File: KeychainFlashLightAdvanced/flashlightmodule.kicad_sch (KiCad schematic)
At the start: 4 parts, among them SW1 SW_DPST_x2

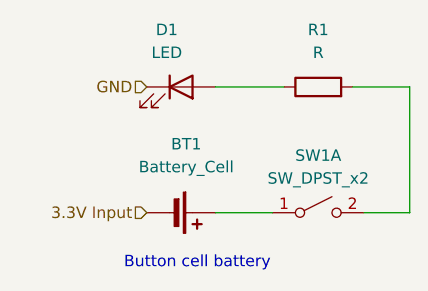
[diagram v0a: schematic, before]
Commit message: cleanup
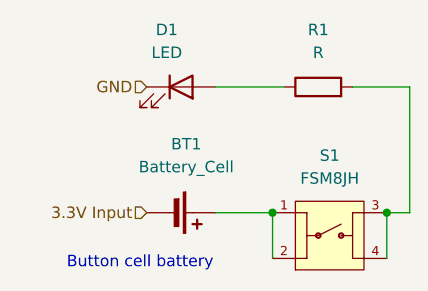
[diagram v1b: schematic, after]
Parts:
- removed SW1: SW_DPST_x2, Button_Switch_THT:SW_Tactile_Straight_KSA0Axx1LFTR, symbol Switch:SW_DPST_x2
- added S1: FSM8JH, FSM8JH:SW_FSM8JH, symbol FSM8JH:FSM8JH
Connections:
- net at BT1.1 (+): now also S1.1, S1.2
- net at R1.2: now also S1.3, S1.4
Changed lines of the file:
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@@
     (comment 1 "Made By: Casper Tak")
   )
+  (junction (at 156.21 106.68) (diameter 0) (color 0 0 0 0)
+  )
+  (junction (at 168.91 106.68) (diameter 0) (color 0 0 0 0)
+  )
   (wire (pts (xy 149.86 106.68) (xy 156.21 106.68))
+    (stroke (width 0) (type default))
+  )
+  (wire (pts (xy 168.91 106.68) (xy 168.91 111.76))
     (stroke (width 0) (type default))
   )
@@
     (stroke (width 0) (type default))
   )
+  (wire (pts (xy 156.21 106.68) (xy 156.21 111.76))
+    (stroke (width 0) (type default))
+  )
   (wire (pts (xy 171.45 92.71) (xy 171.45 106.68))
     (stroke (width 0) (type default))
   )
-  (wire (pts (xy 171.45 106.68) (xy 166.37 106.68))
+  (wire (pts (xy 171.45 106.68) (xy 168.91 106.68))
     (stroke (width 0) (type default))
   )
@@
     (stroke (width 0) (type default))
   )
-  (text "Button cell battery" (at 139.7 113.03 0)
+  (text "Button cell battery" (at 133.35 113.03 0)
     (effects (font (size 1.27 1.27)) (justify left bottom))
   )
@@
   (hierarchical_label "GND" (shape input) (at 142.24 92.71 180) (fields_autoplaced)
     (effects (font (size 1.27 1.27)) (justify right))
+  )
+  (symbol (lib_id "FSM8JH:FSM8JH") (at 162.56 109.22 0) (unit 1)
+    (in_bom yes) (on_board yes) (dnp no) (fields_autoplaced)
+    (property "Reference" "S1" (at 162.56 100.33 0)
+      (effects (font (size 1.27 1.27)))
+    )
+    (property "Value" "FSM8JH" (at 162.56 102.87 0)
+      (effects (font (size 1.27 1.27)))
+    )
+    (property "Footprint" "FSM8JH:SW_FSM8JH" (at 162.56 109.22 0)
+      (effects (font (size 1.27 1.27)) (justify bottom) hide)
+    )
+    (property "Datasheet" "" (at 162.56 109.22 0)
+      (effects (font (size 1.27 1.27)) hide)
+    )
+    (property "MF" "TE Connectivity" (at 162.56 109.22 0)
+      (effects (font (size 1.27 1.27)) (justify bottom) hide)
+    )
+    (property "Description" "\nSwitch,Pushbutton,Tactile,SPST,Thru Hole,Vertical,6MM,Black | TE Connectivity FSM8JH\n" (at 162.56 109.22 0)
+      (effects (font (size 1.27 1.27)) (justify bottom) hide)
+    )
+    (property "Package" "None" (at 162.56 109.22 0)
+      (effects (font (size 1.27 1.27)) (justify bottom) hide)
+    )
+    (property "Price" "None" (at 162.56 109.22 0)
+      (effects (font (size 1.27 1.27)) (justify bottom) hide)
+    )
+    (property "Check_prices" "https://www.snapeda.com/parts/FSM8JH/TE+Connectivity+ALCOSWITCH+Switches/view-part/?ref=eda" (at 162.56 109.22 0)
+      (effects (font (size 1.27 1.27)) (justify bottom) hide)
+    )
+    (property "STANDARD" "MANUFACTURER RECOMMENDATIONS" (at 162.56 109.22 0)
+      (effects (font (size 1.27 1.27)) (justify bottom) hide)
+    )
+    (property "PARTREV" "C10" (at 162.56 109.22 0)
+      (effects (font (size 1.27 1.27)) (justify bottom) hide)
+    )
+    (property "SnapEDA_Link" "https://www.snapeda.com/parts/FSM8JH/TE+Connectivity+ALCOSWITCH+Switches/view-part/?ref=snap" (at 162.56 109.22 0)
+      (effects (font (size 1.27 1.27)) (justify bottom) hide)
+    )
+    (property "MP" "FSM8JH" (at 162.56 109.22 0)
+      (effects (font (size 1.27 1.27)) (justify bottom) hide)
+    )
+    (property "Availability" "In Stock" (at 162.56 109.22 0)
+      (effects (font (size 1.27 1.27)) (justify bottom) hide)
+    )
+    (property "MANUFACTURER" "TE CONNECTIVITY" (at 162.56 109.22 0)
+      (effects (font (size 1.27 1.27)) (justify bottom) hide)
+    )
+    (pin "1")
+    (pin "2")
+    (pin "3")
+    (pin "4")
+    (instances
+      (project "KeychainFlashLightAdvanced"
+        (path "/30398b8a-8fed-4ca8-b3cc-b1f61d914000/10723c4f-449e-4ad5-9164-0f599a2c215f"
+          (reference "S1") (unit 1)
+        )
+      )
+    )
   )
   (symbol (lib_id "Device:LED") (at 146.05 92.71 0) (unit 1)
@@
         )
       )
-    )
-  )
-  (symbol (lib_id "Switch:SW_DPST_x2") (at 161.29 106.68 0) (unit 1)
-    (in_bom yes) (on_board yes) (dnp no) (fields_autoplaced)
-    (property "Reference" "SW1" (at 161.29 100.33 0)
-      (effects (font (size 1.27 1.27)))
-    )
-    (property "Value" "SW_DPST_x2" (at 161.29 102.87 0)
-      (effects (font (size 1.27 1.27)))
-    )
-    (property "Footprint" "Button_Switch_THT:SW_Tactile_Straight_KSA0Axx1LFTR" (at 161.29 106.68 0)
-      (effects (font (size 1.27 1.27)) hide)
-    )
-    (property "Datasheet" "~" (at 161.29 106.68 0)
-      (effects (font (size 1.27 1.27)) hide)
-    )
-    (pin "1")
-    (pin "2")
-    (pin "3")
-    (pin "4")
-    (instances
-      (project "KeychainFlashLightAdvanced"
-        (path "/30398b8a-8fed-4ca8-b3cc-b1f61d914000"
-          (reference "SW1") (unit 1)
-        )
-        (path "/30398b8a-8fed-4ca8-b3cc-b1f61d914000/10723c4f-449e-4ad5-9164-0f599a2c215f"
-          (reference "SW1") (unit 1)
-        )
-      )
